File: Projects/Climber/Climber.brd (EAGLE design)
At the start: 59 x 65.8 mm, 14 parts, among them M1 VNH5019, M2 D24V10FX, U1 NRF52840-DONGLE, U2 BSS138BKW

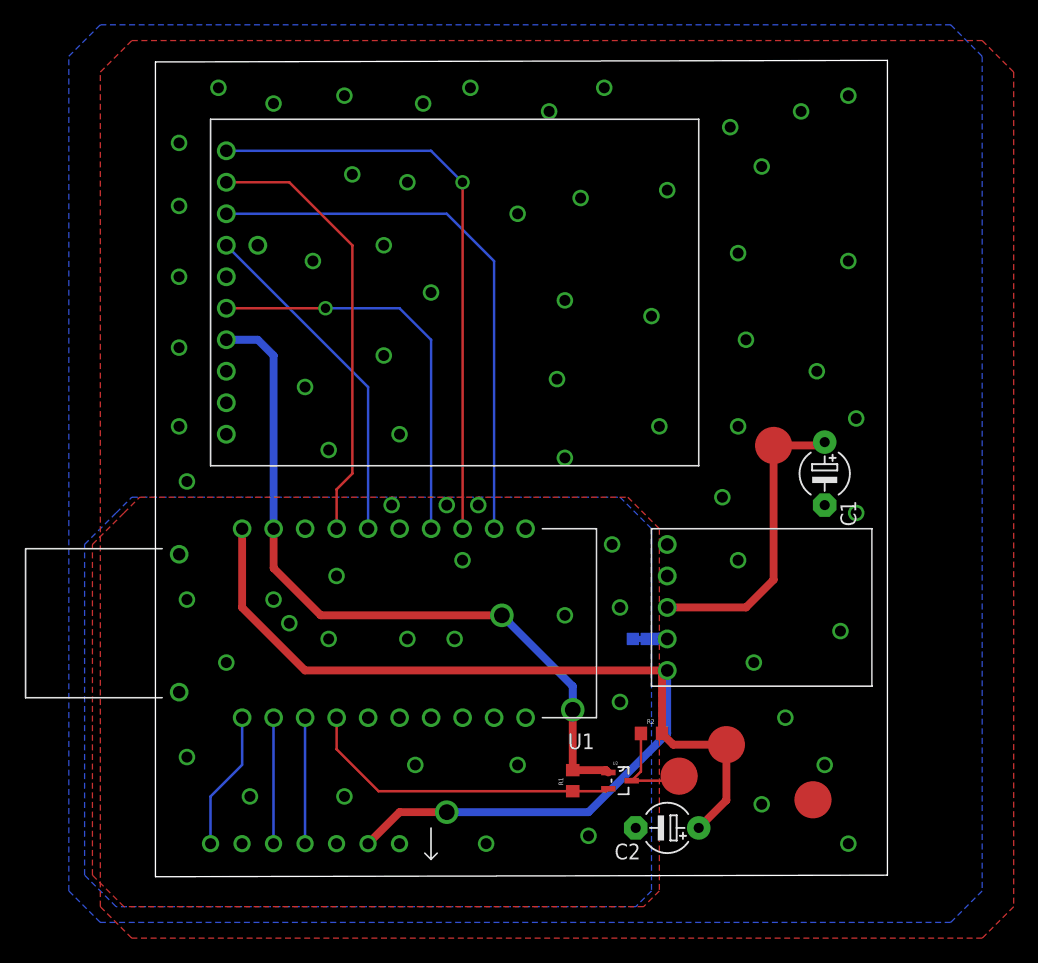
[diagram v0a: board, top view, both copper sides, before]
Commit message: Updated stravaV3 Updated Climber
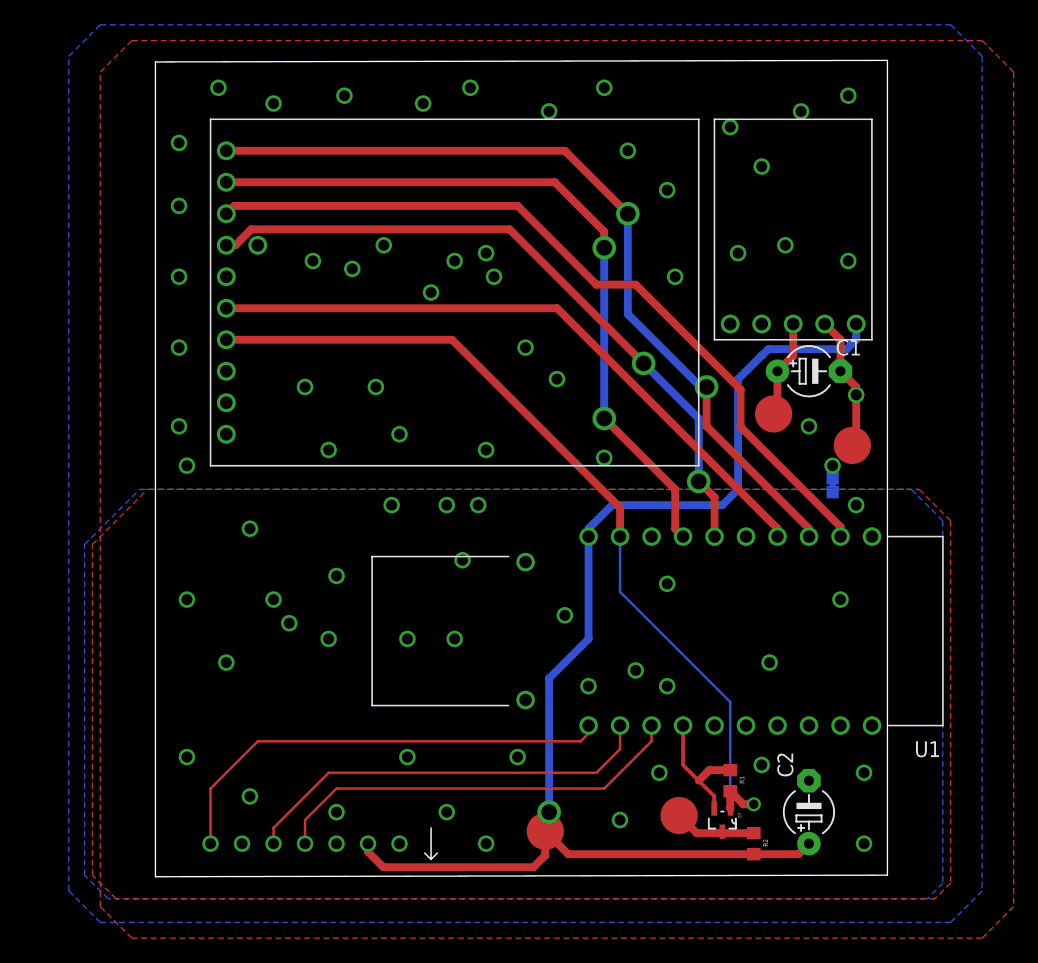
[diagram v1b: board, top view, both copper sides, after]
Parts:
- moved M2 31.8 mm to (57.1, 78.7), turned to 180 degrees
- moved NEO1 28.8 mm to (56.5, 67.9)
- moved U1 27.9 mm to (58.4, 46.4)
- moved U$10 19.8 mm to (55.2, 66.7), turned to 270 degrees
- moved 5V 16.2 mm to (31.8, 36.8)
- moved R1 12.7 mm to (47.0, 41.9), turned to 270 degrees
- moved R2 12.1 mm to (48.9, 36.8), turned to 270 degrees
- moved C2 11.5 mm to (53.3, 39.4), turned to 90 degrees
- moved U2 8.84 mm to (46.4, 38.7), turned to 270 degrees
- moved C1 8.35 mm to (53.3, 74.9), turned to 0 degrees
- moved NEO 3.17 mm to (42.5, 38.1)
- moved VIN 2.54 mm to (50.2, 70.5)
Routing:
- net M1_CS: track 27.6 -> 55.0 mm, vias 0 -> 2
- net GPIO1: track 11.2 -> 37.4 mm
- net M1_ENA/DIAGA: track 35.7 -> 59.4 mm, vias 0 -> 2
- net SCL: track 10.2 -> 33.7 mm
- net SDA: track 10.2 -> 33.7 mm
- net M1_INB: track 32.8 -> 52.5 mm, vias 1 -> 0
- net M1_INA: track 48.0 -> 66.9 mm, vias 1 -> 2
- net M1_PWM: track 44.8 -> 63.1 mm
- net 12V: track 24.6 -> 7.91 mm
- net NEO_LV: track 25.9 -> 10.6 mm
- net VDD: track 59.3 -> 69.9 mm, vias 2 -> 1
- net PWR_GND: track 2.67 -> 12.0 mm, vias 49 -> 41
- net VDD_5V: track 94.1 -> 100.4 mm
- net NEO_HV: track 8.10 -> 6.78 mm

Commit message: Order @ Boktech
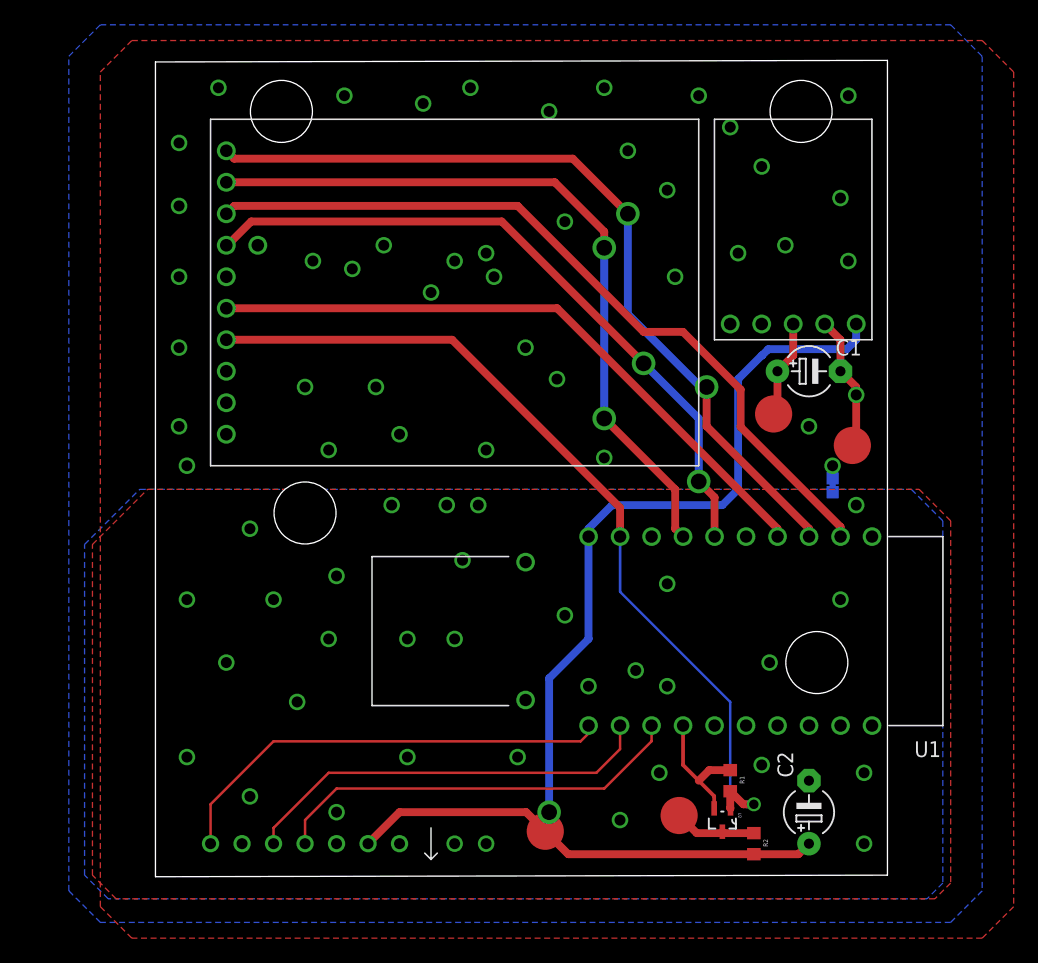
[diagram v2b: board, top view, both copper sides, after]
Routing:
- net VDD_5V: track 100.4 -> 98.6 mm
- net GPIO1: track 37.4 -> 36.7 mm
- net M1_CS: track 55.0 -> 55.5 mm
- net PWR_GND: vias 41 -> 42
